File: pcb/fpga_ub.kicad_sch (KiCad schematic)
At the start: 1 part

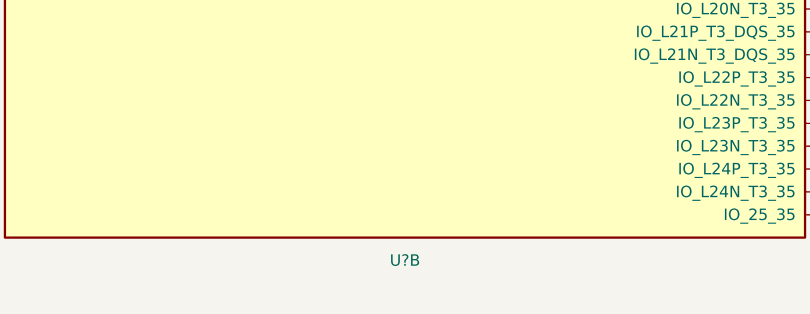
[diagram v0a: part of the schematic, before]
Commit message: kicad said I needed to save
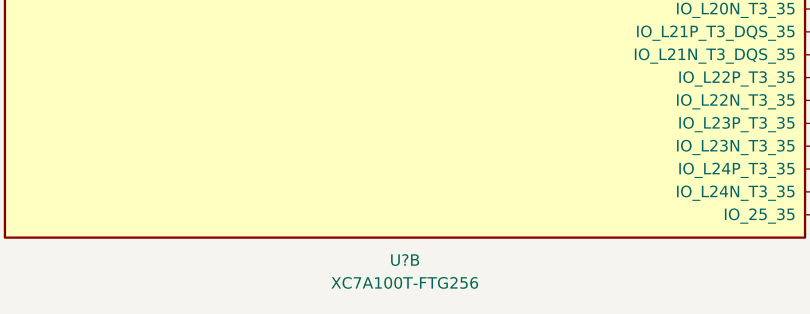
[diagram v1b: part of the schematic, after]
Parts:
- U?: value (none) -> XC7A100T-FTG256
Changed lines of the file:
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@@
     (in_bom yes) (on_board yes) (fields_autoplaced)
     (property "Reference" "U?" (id 0) (at 93.98 179.07 0))
-    (property "Value" "" (id 1) (at 93.98 181.61 0))
+    (property "Value" "XC7A100T-FTG256" (id 1) (at 93.98 181.61 0))
     (property "Footprint" "" (id 2) (at 93.98 102.87 0)
       (effects (font (size 1.27 1.27)) hide)
